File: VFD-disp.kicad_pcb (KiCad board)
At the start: 4 copper layers, 99.6 x 65.5 mm, 101 parts, among them J1 USB_C_Receptacle_USB2.0_14P, J2 Conn_02x03_Odd_Even, J4 Conn_02x03_Odd_Even, J5 Conn_02x03_Odd_Even, J6 Conn_02x03_Odd_Even, Q1 Q_NMOS_GDS, Q2 Q_NMOS_GDS, SW1 SW_SPST, U1 ESP32-C6-WROOM-1, U10 TXS0104EPW, U11 MAX811TEUS-T, U12 MCP4728, U2 FUSB302B01MPX, U3 LM1117DT-3.3, U4 MCP1416, U5 LM2576HVS-ADJ, U6 MAX1771xSA, U7 LM2576HVS-ADJ, U9 FM24C64B, Y1 Crystal

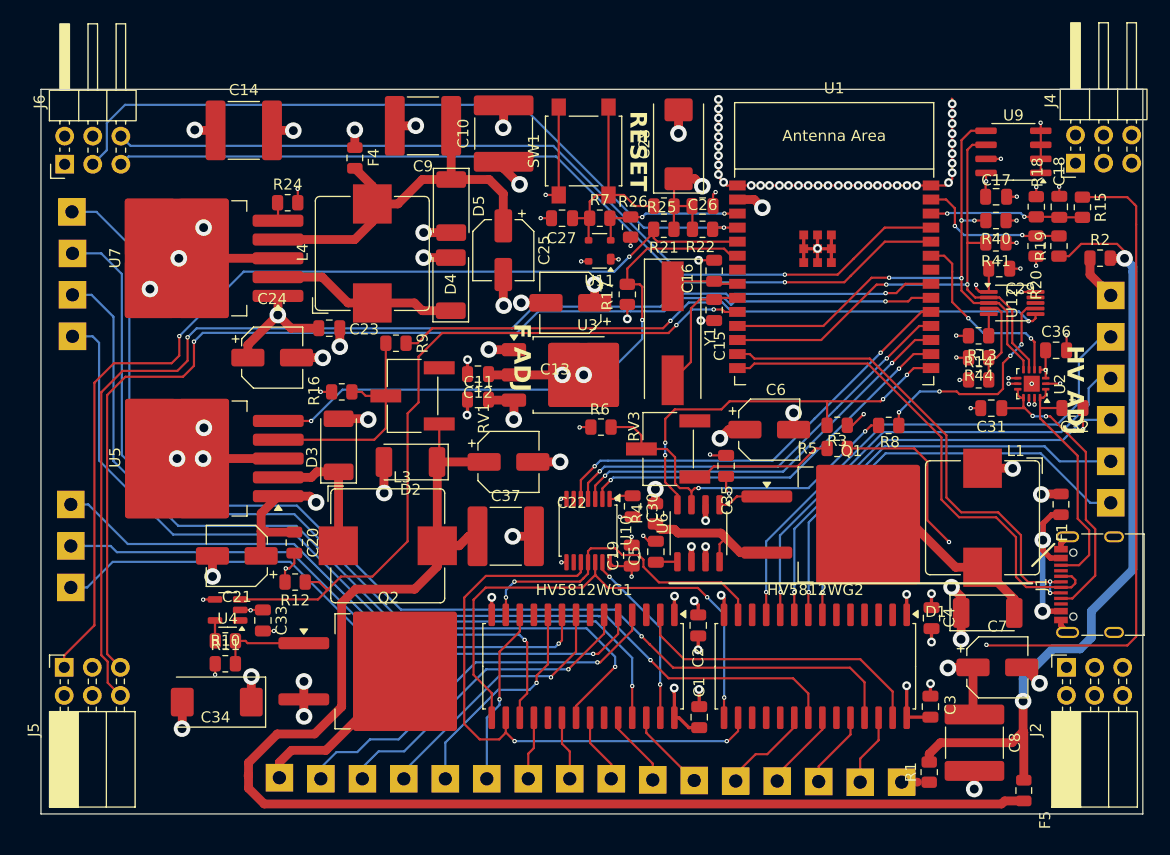
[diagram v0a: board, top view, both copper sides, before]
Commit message: Finish pcb
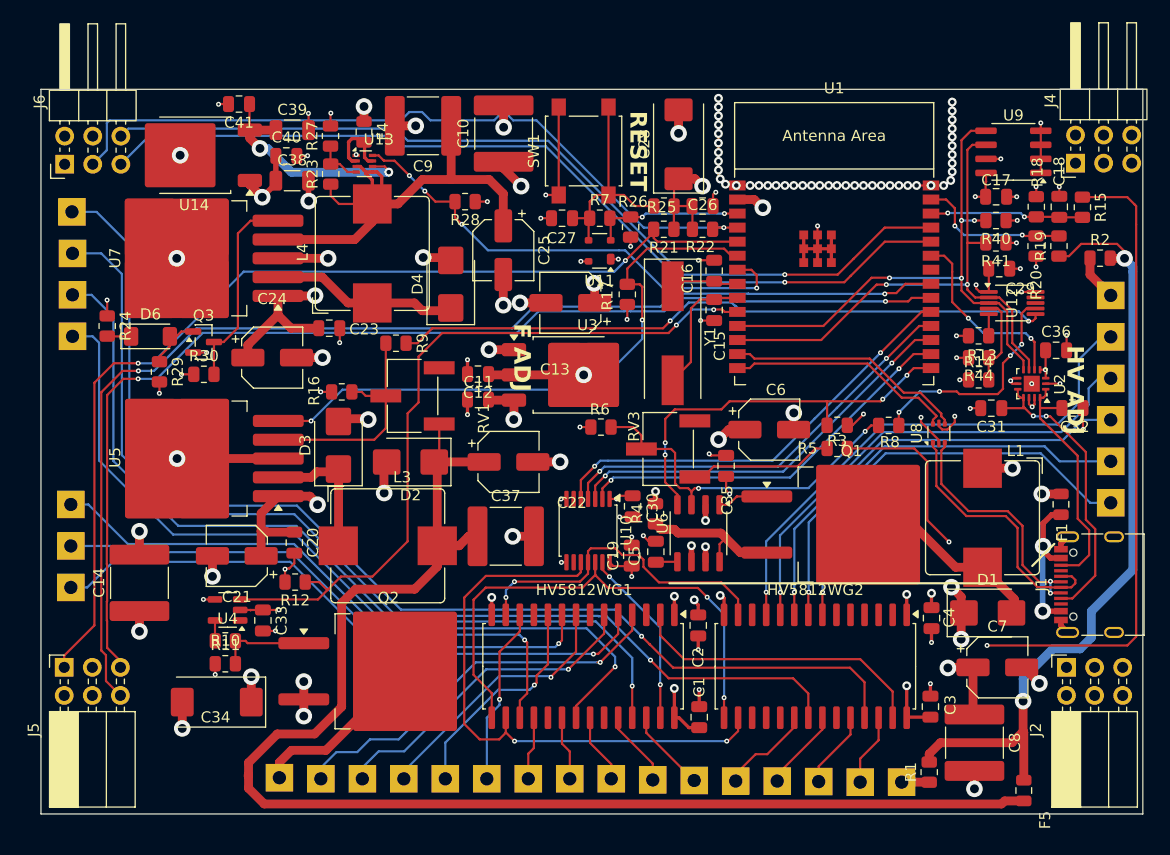
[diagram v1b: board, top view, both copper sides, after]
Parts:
- removed D5: D_Zener, Diode_SMD:D_MELF
- added C38: 10uF, Capacitor_SMD:C_1206_3216Metric, F.Cu at (61.8, 197.5)
- added C39: 10uF, Capacitor_SMD:C_1206_3216Metric, F.Cu at (61.8, 192.9)
- added C40: C, Capacitor_SMD:C_0805_2012Metric, F.Cu at (61.3, 195.3)
- added C41: C, Capacitor_SMD:C_0805_2012Metric, F.Cu at (57.0, 190.6)
- added D6: BZV55B7V5, Diode_SMD:D_MiniMELF, F.Cu at (49.0, 211.6)
- added Q3: Q_NPN_BEC, Package_TO_SOT_SMD:SOT-23, F.Cu at (53.8, 212.1)
- added R23: R, Resistor_SMD:R_0805_2012Metric, F.Cu at (65.3, 196.9)
- added R27: R, Resistor_SMD:R_0805_2012Metric, F.Cu at (65.3, 193.5)
- added R28: R, Resistor_SMD:R_0805_2012Metric, F.Cu at (77.4, 199.4)
- added R29: R, Resistor_SMD:R_0805_2012Metric, F.Cu at (49.8, 214.8)
- added R30: R, Resistor_SMD:R_0805_2012Metric, F.Cu at (53.8, 215.0)
- added U13: TPS2116DRL, Package_TO_SOT_SMD:SOT-583-8, F.Cu at (68.3, 196.0)
- added U14: KF50BDT, Package_TO_SOT_SMD:TO-252-2, F.Cu at (52.9, 195.2)
- added U8: USBLC6-2P6, Package_TO_SOT_SMD:SOT-666, F.Cu at (120.3, 220.3)
- D1, D2, D3, D4: footprint Diode_SMD:D_MELF -> Diode_SMD:D_SMB
- moved C14 42.0 mm to (48.0, 233.9), turned to 90 degrees
- moved R24 19.8 mm to (45.1, 210.6), turned to -90 degrees
- moved F4 2.49 mm to (68.3, 193.1)
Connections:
- C25 pad 1: Net-(D5-K) -> Net-(U13-MODE)
- C9 pad 1: Net-(D5-K) -> Net-(U13-MODE)
- F4 pad 1: Net-(D5-K) -> Net-(F4-Pad1)
- L4 pad 2: Net-(D5-K) -> Net-(U13-MODE)
- R24 pad 1: Net-(U7-~{ON}/OFF) -> VBUS
- R24 pad 2: GND -> Net-(D6-K)
- U1 pad 13: USB_D- -> PRE_USB_D-
- U1 pad 14: USB_D+ -> PRE_USB_D+
- U1 pad 7: unconnected-(U1-MTDO/GPIO7-Pad7) -> VBUS_ABOVE_TRESHOLD
- U7 pad 4: Net-(D5-K) -> Net-(U13-MODE)
- U7 pad 5: Net-(U7-~{ON}/OFF) -> Net-(Q3-C)
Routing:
- net Net-(U13-MODE): track 0.00 -> 45.6 mm
- net VBUS_ABOVE_TRESHOLD: track 0.00 -> 43.6 mm, vias 0 -> 4
- net Net-(D5-K): track 35.7 -> 0.00 mm
- net USB_D-: track 45.2 -> 22.5 mm
- net USB_D+: track 46.4 -> 24.4 mm
- net PRE_USB_D-: track 0.00 -> 21.7 mm
- net Net-(U13-VIN2): track 0.00 -> 21.1 mm, vias 0 -> 2
- net PRE_USB_D+: track 0.00 -> 21.0 mm
- net Net-(Q3-C): track 0.00 -> 18.2 mm
- net VBUS: track 37.1 -> 49.7 mm, vias 9 -> 12
- net Net-(F4-Pad1): track 0.00 -> 6.32 mm
- net +3.3V: track 46.3 -> 52.2 mm
- net GND: track 179.3 -> 184.4 mm, vias 112 -> 123
- net Net-(D6-A): track 0.00 -> 4.97 mm
- net Net-(U13-PR1): track 0.00 -> 4.22 mm
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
